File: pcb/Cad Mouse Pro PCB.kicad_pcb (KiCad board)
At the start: 2 copper layers, 69.8 x 69.8 mm, 25 parts, among them J1 reset, J2 encoder, J3 Key2, J4 Key1, J5 LED, U1 ProMicro

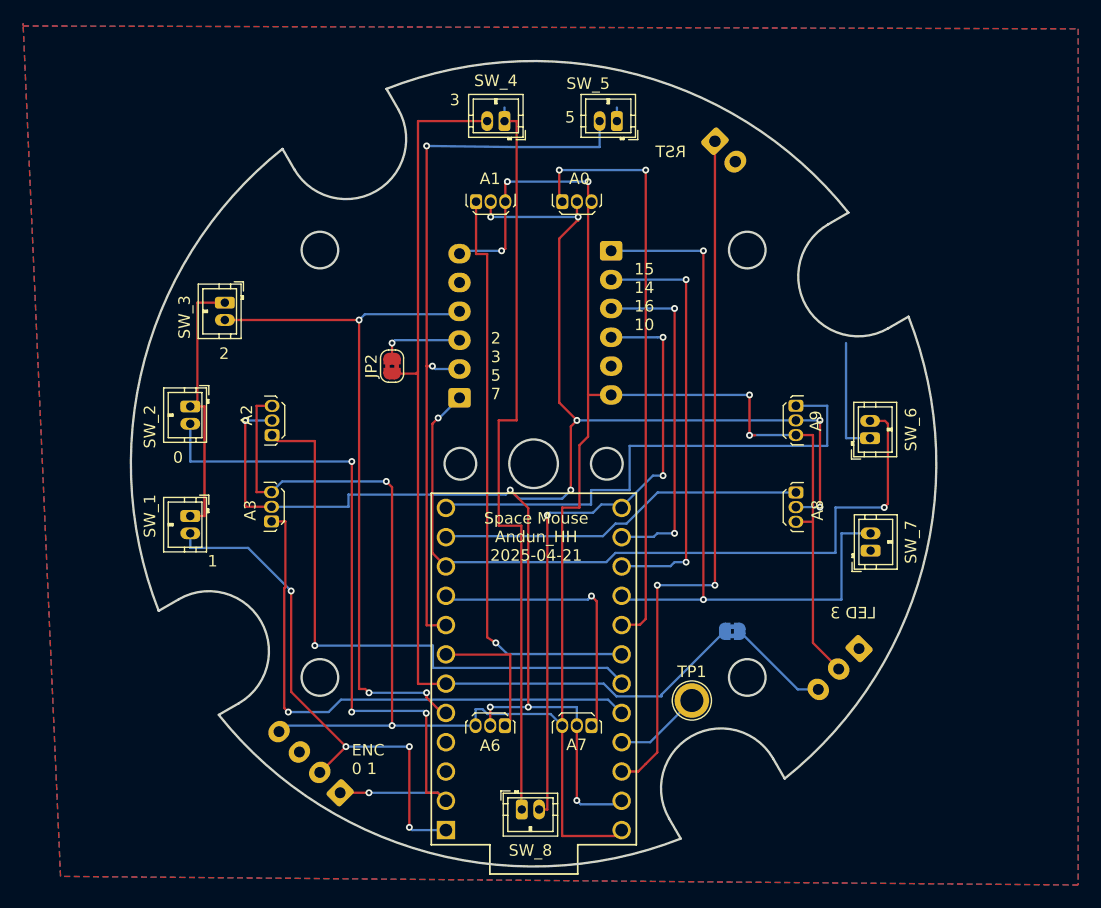
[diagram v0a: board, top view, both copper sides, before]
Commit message: include odb and gerber files. untested!
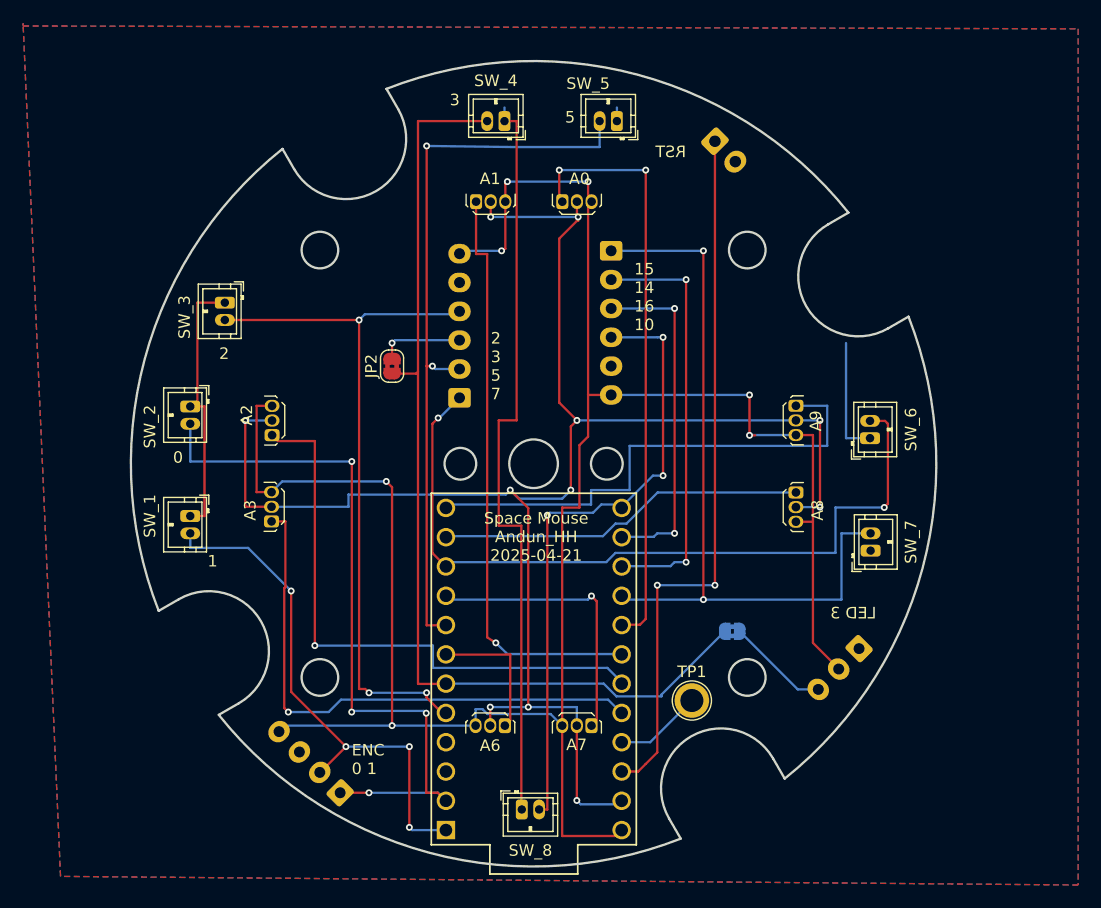
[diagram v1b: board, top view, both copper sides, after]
